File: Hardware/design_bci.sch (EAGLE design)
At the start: 11 parts, among them IC1 AD623N

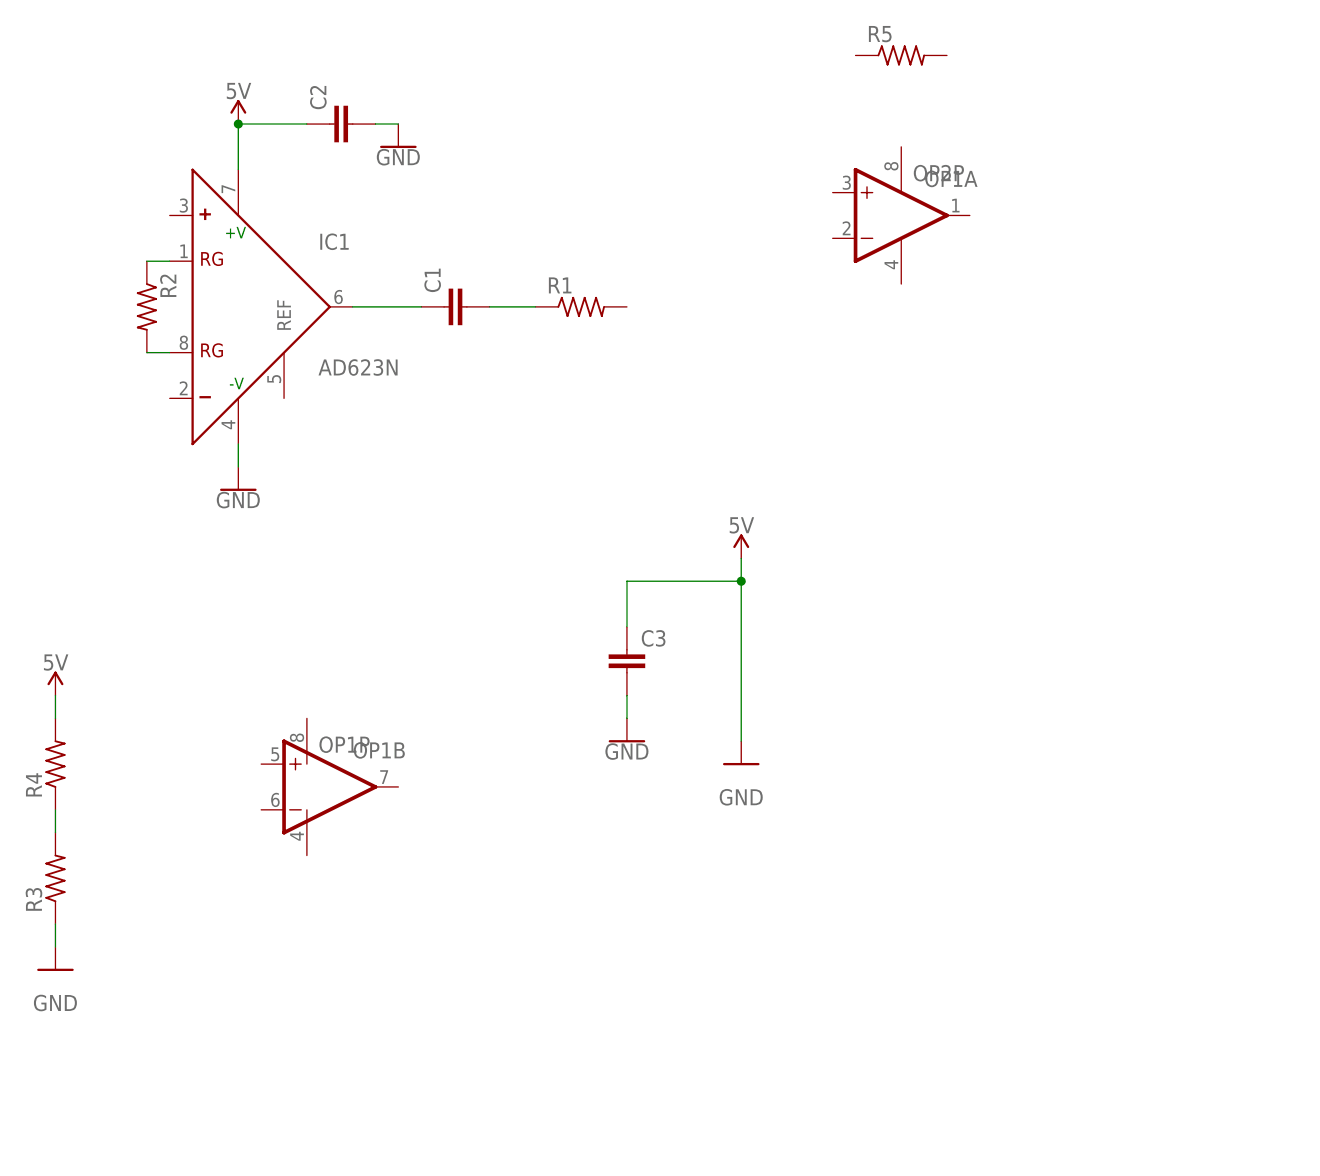
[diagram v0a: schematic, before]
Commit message: updated
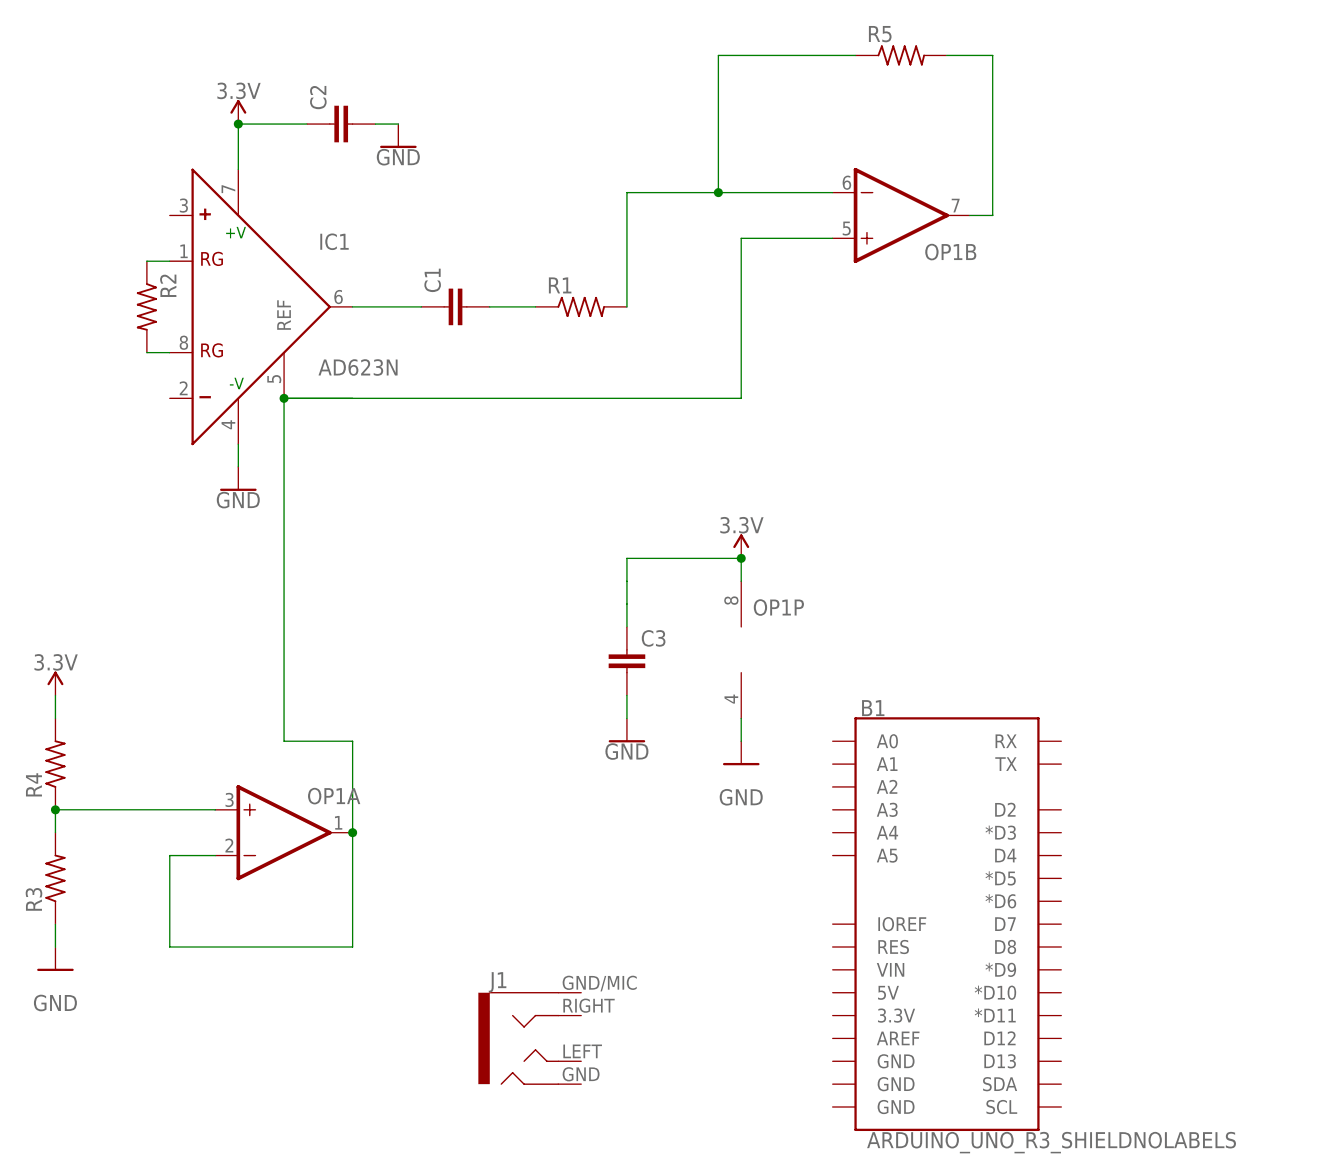
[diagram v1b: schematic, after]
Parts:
- removed OP2: (no value), LinnesLab-AnalogIC:OP-DUALR
- added B1: ARDUINO_UNO_R3_SHIELDNOLABELS, LinnesLab-Microcontrollers:ARDUINO_UNO_R3_SHIELDNOLABELS
- added J1: (no value), LinnesLab-Connectors:AUDIO_JACK_TRRSSMD_RA
- OP1: device LinnesLab-AnalogIC:OP-DUALR -> LinnesLab-AnalogIC:OP-DUALMCP6002R
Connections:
- removed net 5V: C2.1, C3.1, IC1.+V, R4.2
- new net 3.3V: C2.1, C3.1, IC1.+V, OP1P.V+, R4.2
- new net N$6: IC1.REF, OP1A.-IN, OP1A.OUT, OP1B.+IN
- new net N$7: OP1B.-IN, R1.2, R5.1
- new net N$8: OP1B.OUT, R5.2
- net GND: now also OP1P.V-
- net N$3: now also OP1A.+IN
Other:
- moved on the sheet: OP1A, OP1B, OP1P
